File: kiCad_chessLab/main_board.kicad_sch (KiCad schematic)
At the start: 18 parts, among them IC1 ESP32-C6-WROOM-1-N8, J1 TYPE-C-31-M-12, J2 PWR, J3 DATA, U2 74HC138

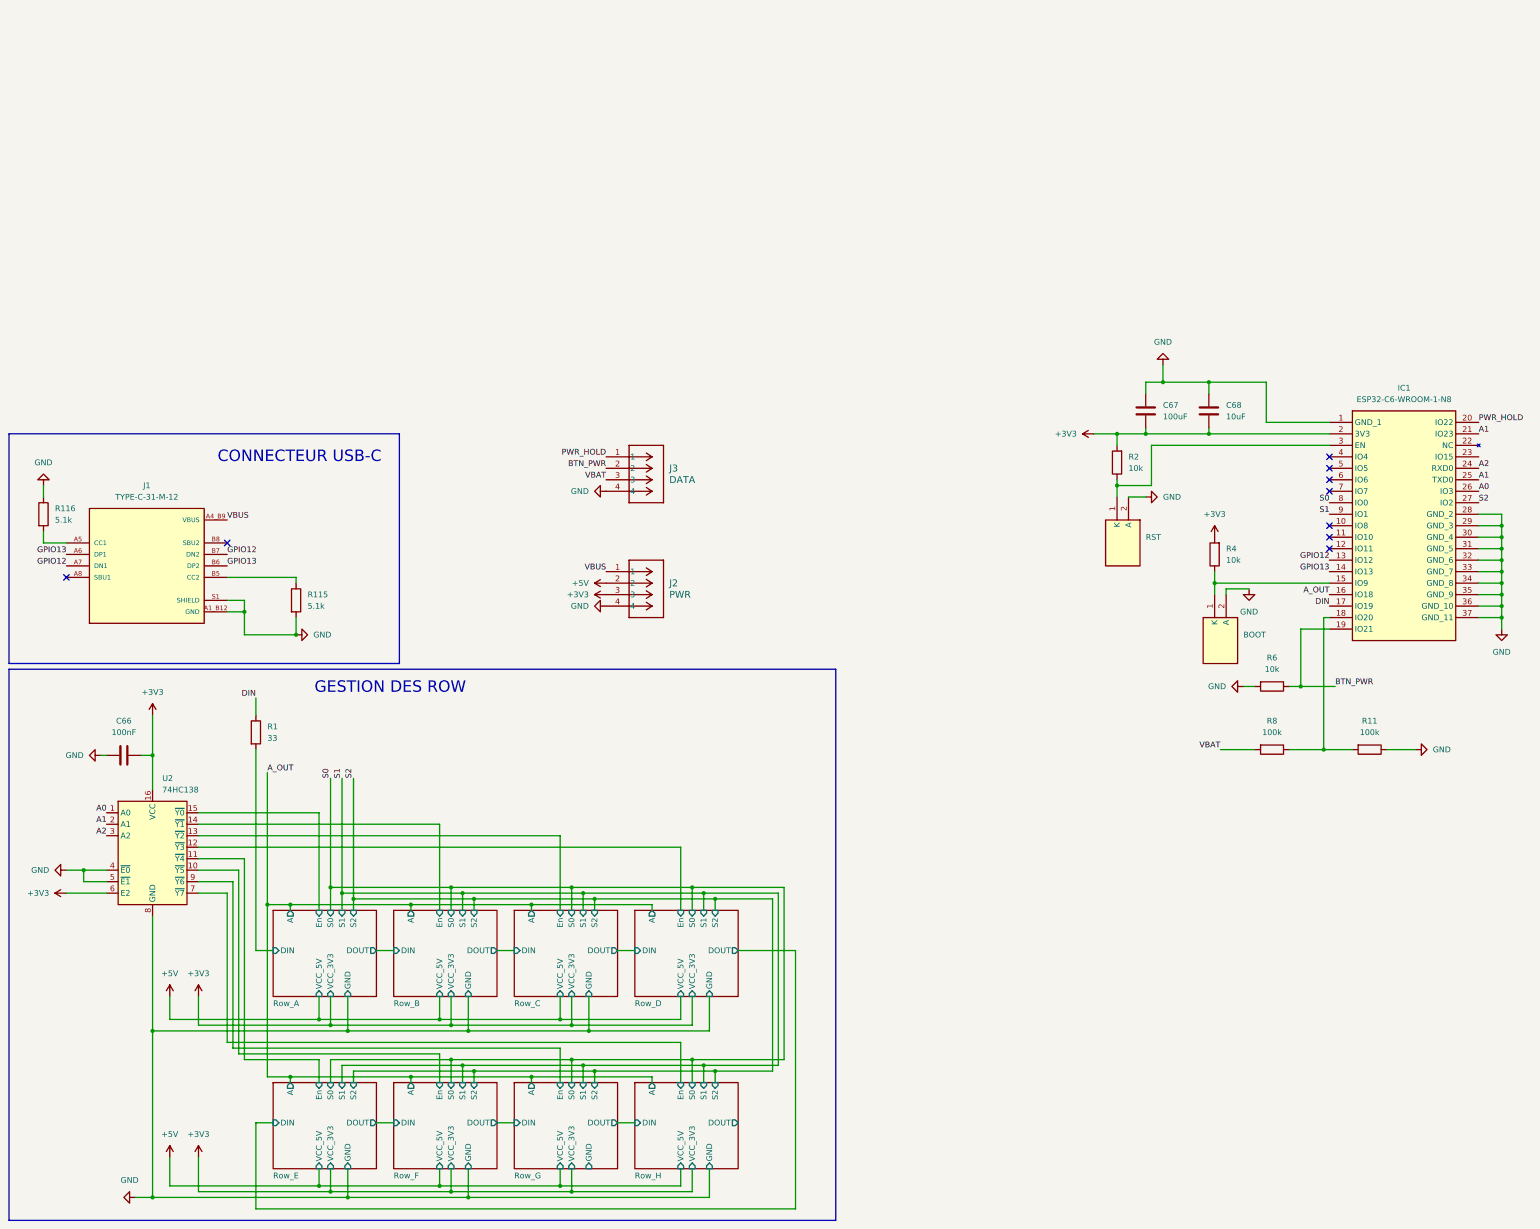
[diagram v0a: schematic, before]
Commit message: Complete Schematics
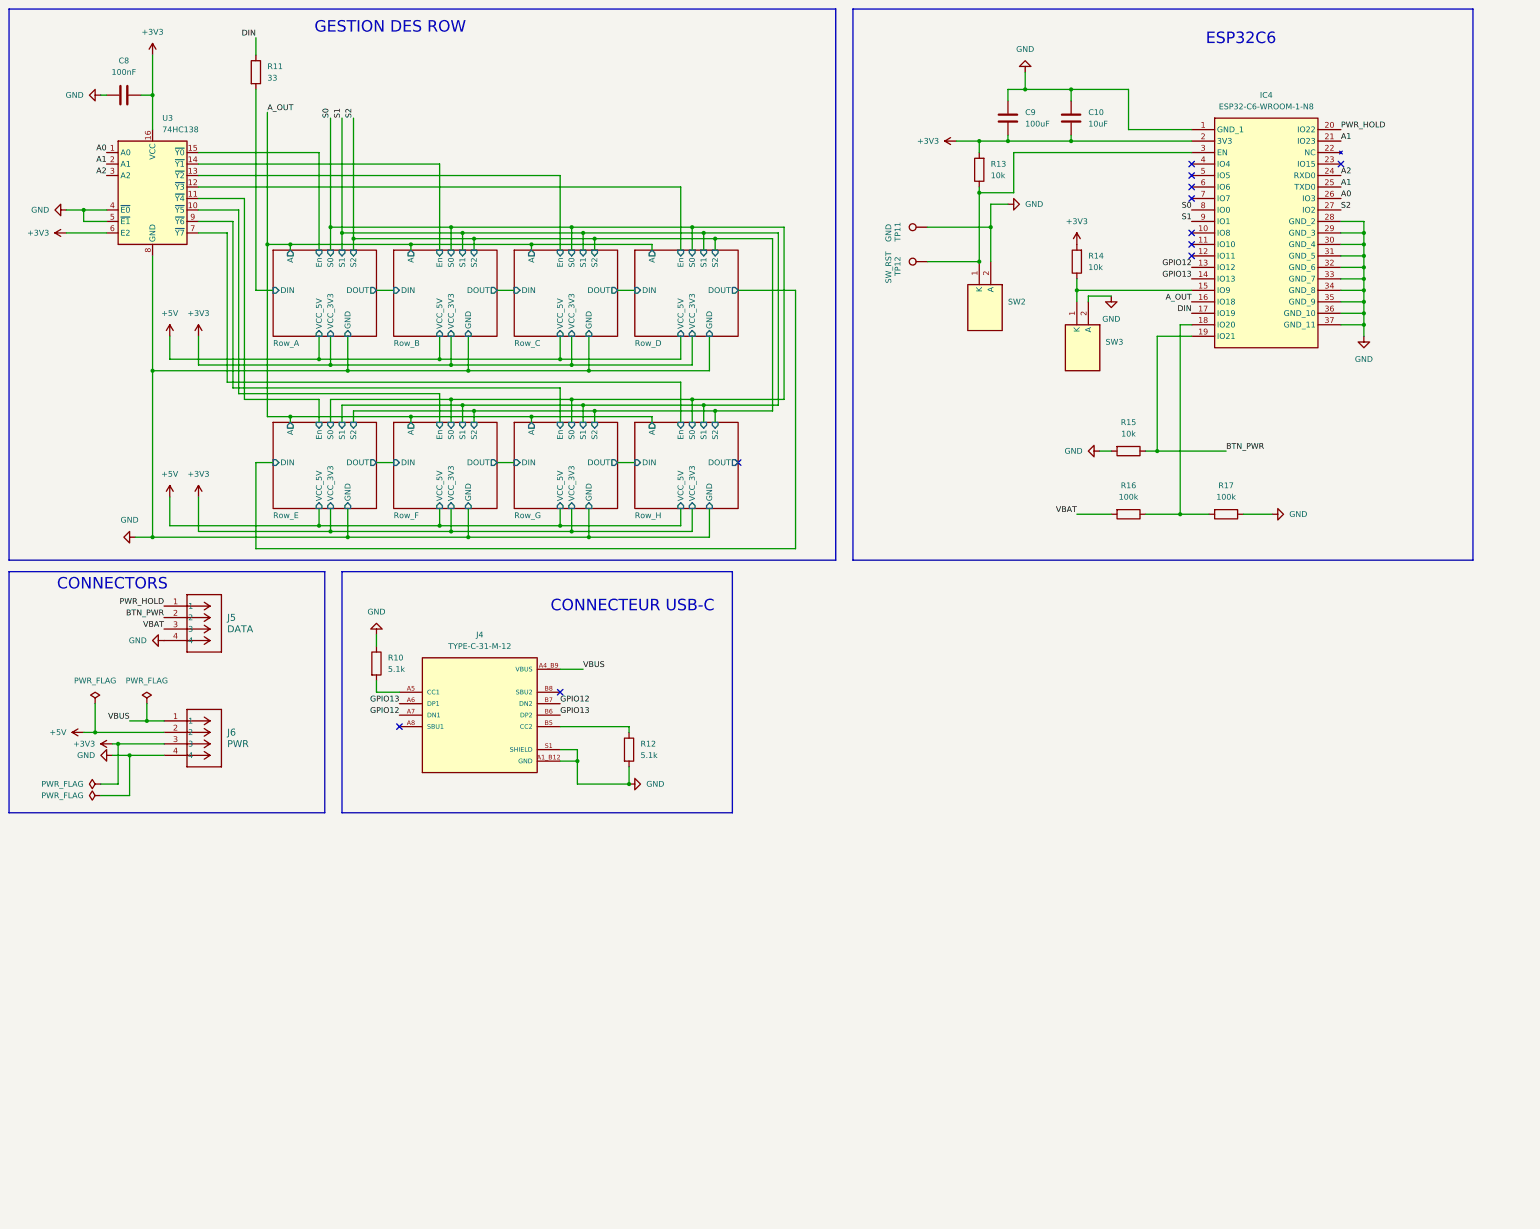
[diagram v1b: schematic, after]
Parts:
- added TP11: GND, TestPoint:TestPoint_Plated_Hole_D2.0mm, symbol Connector:TestPoint
- added TP12: SW_RST, TestPoint:TestPoint_Plated_Hole_D2.0mm, symbol Connector:TestPoint
- SW2: renamed from RST; value B3U-1000P -> RST
- SW3: renamed from BOOT; value B3U-1000P -> BOOT
- renumbered C68 to C10, C66 to C8, C67 to C9, IC1 to IC4, J1 to J4, J3 to J5, J2 to J6, R116 to R10, R1 to R11, R115 to R12, R2 to R13, R4 to R14, R6 to R15, R8 to R16, R11 to R17, U2 to U3
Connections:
- net GND: now also TP11.1
- net at IC4.3 (EN), R13.1, SW2.1 (K): now also TP12.1
- no-connect marks 9 -> 11
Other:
- note added: "CONNECTORS"
- note added: "ESP32C6"
- moved on the sheet: C10, C8, C9, IC4, J4, J5, J6, R10, R11, R12, R13, R14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

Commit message: PCB SetUp
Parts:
- J4: footprint TYPE-C-31-M-12:HRO_TYPE-C-31-M-12 -> chessLab-footprints:HRO_TYPE-C-31-M-12
- J5, J6: footprint CONN4_1048_KEY -> Connector_JST:JST_XH_B4B-XH-A_1x04_P2.50mm_Vertical
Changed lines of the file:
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@@
 			)
 		)
-		(property "Footprint" "CONN4_1048_KEY"
+		(property "Footprint" "Connector_JST:JST_XH_B4B-XH-A_1x04_P2.50mm_Vertical"
 			(at 48.26 147.32 0)
 			(effects
@@
 			)
 		)
-		(property "Footprint" "CONN4_1048_KEY"
+		(property "Footprint" "Connector_JST:JST_XH_B4B-XH-A_1x04_P2.50mm_Vertical"
 			(at 48.26 172.72 0)
 			(effects
@@
 			)
 		)
-		(property "Footprint" "TYPE-C-31-M-12:HRO_TYPE-C-31-M-12"
+		(property "Footprint" "chessLab-footprints:HRO_TYPE-C-31-M-12"
 			(at 118.11 171.45 0)
 			(effects
